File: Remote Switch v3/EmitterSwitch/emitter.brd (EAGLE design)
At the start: 31.5 x 41.9 mm, 29 parts, among them IC2 STM8L101F2, Q1 MMBT3906LT1SMD

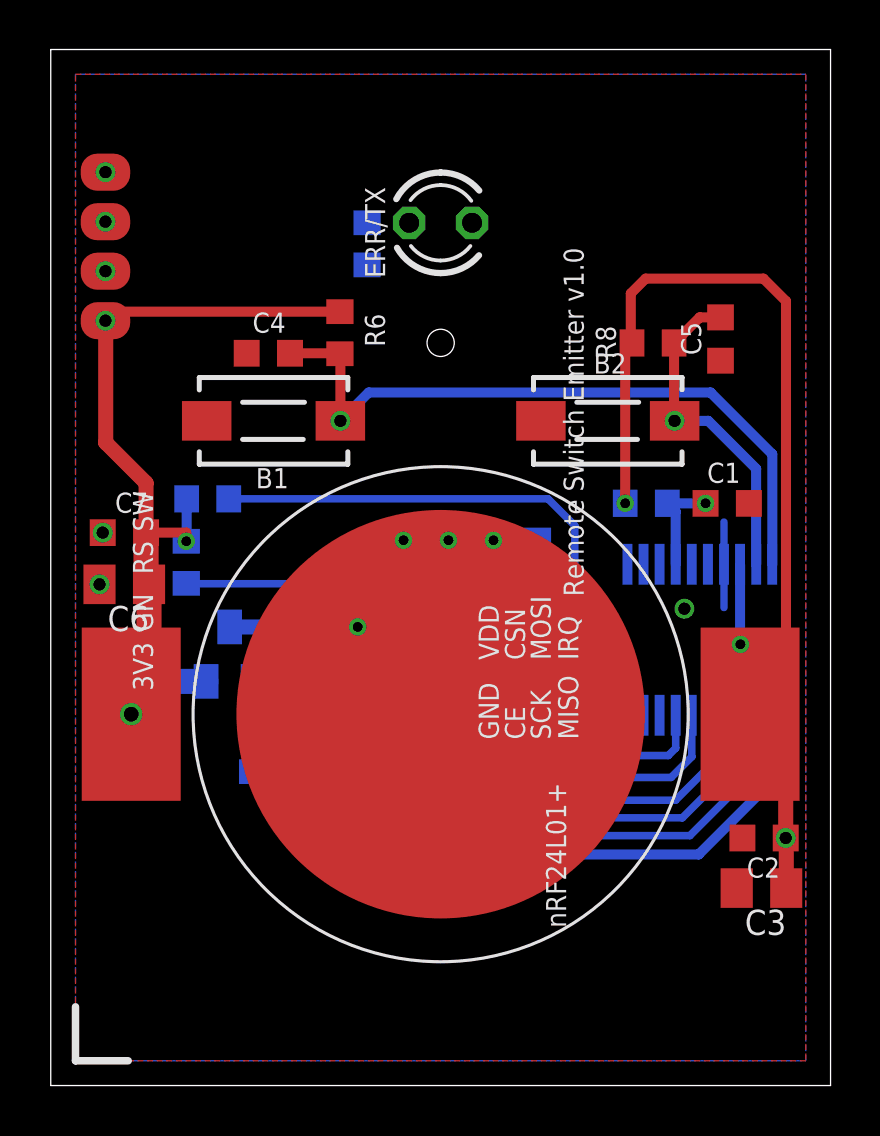
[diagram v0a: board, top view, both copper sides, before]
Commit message: PCB work
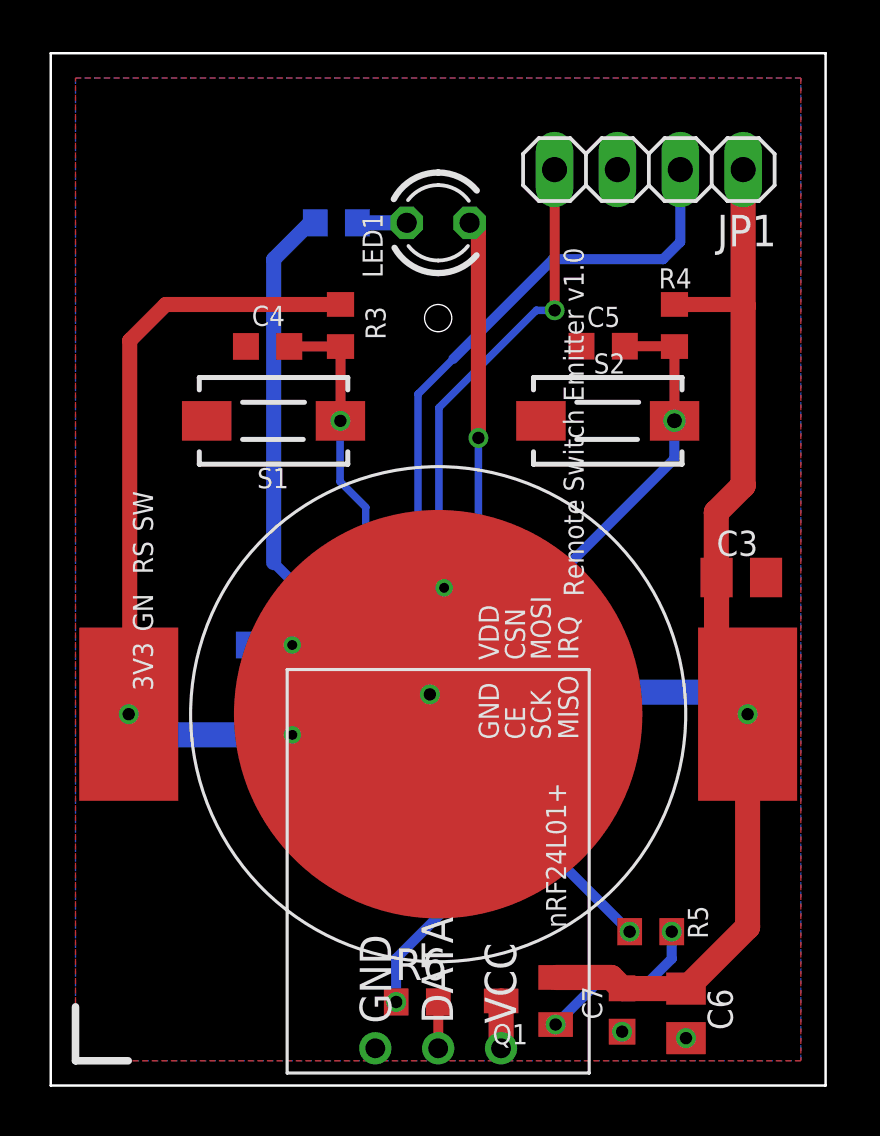
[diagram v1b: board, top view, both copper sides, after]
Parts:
- removed ERR/TX: (no value), led:LED3MM
- removed R10: 1K, resistor:R0603
- removed R11, R12, R7, R8, R9: 10k, resistor:R0603
- removed SIG_+3V1, SIG_GND, SIG_RST, SIG_SWIM: CON_PAD, componente_RFSwitch:SMD_PAD
- removed U$1: MINI_NRF24L01+, comp_RFSwitch_v2:MINI_NRF24L01+
- removed U$2: CR2032_HOLDER_BC-2003, comp_RFSwitch_v2:CR2032_HOLDER_BC-2003
- added IC1: STM8L101F2, comp_RFSwitch_v2:TSSOP20
- added JP1: (no value), pinhead:1X04
- added LED1: (no value), led:LED3MM
- added R2: 10k, resistor:R0603
- added S1: DTSM-3, switch-tact:DTSM-3
- B1: value DTSM-3 -> (none); device switch-tact:DTSM-3 -> comp_RFSwitch_v2:CR2032_HOLDER_BC-2003
- IC2: value STM8L101F2 -> RFM85W; device comp_RFSwitch_v2:TSSOP20 -> comp_RFSwitch_v3:RFM85W_CON
- R5, R6: value 10k -> 1K
- moved C6 28.6 mm to (25.7, 2.92), turned to 270 degrees
- moved C7 27.9 mm to (23.1, 3.05), turned to 270 degrees
- moved R6 27.2 mm to (14.8, 3.38), turned to 0 degrees
- moved R4 21.9 mm to (25.2, 30.7), flipped to the top
- moved IC2 20.8 mm to (15.7, 0.51), flipped to the top, turned to 0 degrees
- moved C1 19.3 mm to (8.88, 17.8), flipped to the bottom
- moved Q1 18.5 mm to (19.3, 3.42), flipped to the top, turned to 90 degrees
- moved R5 18.0 mm to (24.2, 6.21), flipped to the top, turned to 0 degrees
- moved R3 14.3 mm to (11.7, 30.7), flipped to the top, turned to 90 degrees
- moved B1 13.6 mm to (15.7, 15.0)
- moved C3 12.6 mm to (27.9, 20.5), turned to 0 degrees
- moved C2 10.4 mm to (19.7, 15.0), flipped to the bottom, turned to 270 degrees
- moved C5 4.75 mm to (22.3, 29.9), turned to 180 degrees
- moved R1 1.51 mm to (11.5, 34.9), turned to 0 degrees
- moved C4 0.28 mm to (8.76, 29.9)
- renumbered B2 to S2
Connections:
- removed net N$4: Q1.C, U$1.P_3V3
- removed net NRF_CE: IC2.13, R5.2, U$1.P_CSN
- removed net NRF_CSN: IC2.12, R4.1, U$1.P_CE
- removed net NRF_IRQ: IC2.20, R7.1, U$1.P_IRQ
- removed net NRF_MISO: IC2.17, R9.2, U$1.P_MISO
- removed net NRF_MOSI: IC2.16, R11.2, U$1.P_MOSI
- removed net NRF_ON: IC2.11, R10.1
- removed net NRF_SCK: IC2.15, R12.2, U$1.P_SCK
- new net N$2: IC2.VCC, Q1.C
- new net RFM85_DATA: IC2.DATA, R6.2
- new net RFM85_ON: IC1.11, R5.1
- new net UC_RFM85_DATA: IC1.13, R6.1
- net +3V0: now also B1.POS1, B1.POS2, IC1.8, JP1.1, R2.2; no longer IC2.8, R6.2, R7.2, R8.2, SIG_+3V1.P$1, U$2.P$POS1, U$2.P$POS2
- net BTN1: now also IC1.2, R3.1, S1.2; no longer B1.2, IC2.10, R6.1
- net BTN2: now also IC1.10, R4.1; no longer IC2.9, R8.1
- net GND: now also B1.NEG, IC1.7, IC2.GND, JP1.3, S1.1; no longer B1.1, IC2.7, R11.1, R12.1, R5.1, R9.1, SIG_GND.P$1, U$1.P_GND, U$2.P$NEG
- net LED_ERR_TX1: now also IC1.9, LED1.K; no longer ERR/TX.K, IC2.1
- net LED_ERR_TX2: now also IC1.1; no longer IC2.2
- net N$1: now also LED1.A; no longer ERR/TX.A
- net N$8: now also R5.2; no longer R10.2
- net RST: now also IC1.4, JP1.4, R2.1; no longer IC2.4, R3.1, SIG_RST.P$1
- net SWIM: now also IC1.3, JP1.2; no longer IC2.3, SIG_SWIM.P$1
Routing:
- net NRF_CSN: track 32.1 -> 0.00 mm
- net SWIM: track 0.00 -> 26.6 mm, vias 1 -> 0
- net NRF_ON: track 26.3 -> 0.00 mm
- net RST: track 4.15 -> 28.1 mm
- net NRF_IRQ: track 23.9 -> 0.00 mm
- net NRF_CE: track 22.3 -> 0.00 mm
- net NRF_SCK: track 19.3 -> 0.00 mm
- net LED_ERR_TX2: track 0.00 -> 18.9 mm
- net LED_ERR_TX1: track 0.00 -> 16.9 mm, vias 0 -> 1
- net NRF_MOSI: track 16.6 -> 0.00 mm
- net +3V0: track 82.0 -> 96.8 mm, vias 6 -> 3
- net NRF_MISO: track 14.0 -> 0.00 mm
- net BTN1: track 28.1 -> 14.3 mm
- net UC_RFM85_DATA: track 0.00 -> 9.69 mm, vias 0 -> 1
- net RFM85_ON: track 0.00 -> 8.00 mm, vias 0 -> 1
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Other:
- board size 31.5 x 41.9 mm -> 31.3 x 41.7 mm
